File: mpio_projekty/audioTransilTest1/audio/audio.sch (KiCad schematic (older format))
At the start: 49 parts, among them J1 USB_B, J2 Mini-Fit Jr; 4,2mm, J3 TUEA4F2SOBHT, J4 Conn_02x05, J5 SWD_4pin, Q1 BC817, Q2 BC817, SW1 TACTM-34N-F, U1 STM32F042K6Tx, U2 AP1509-50SG-13, U3 LD1117S33TR, U4 IRLTS2242, U5 AO4616, U6 AO4616

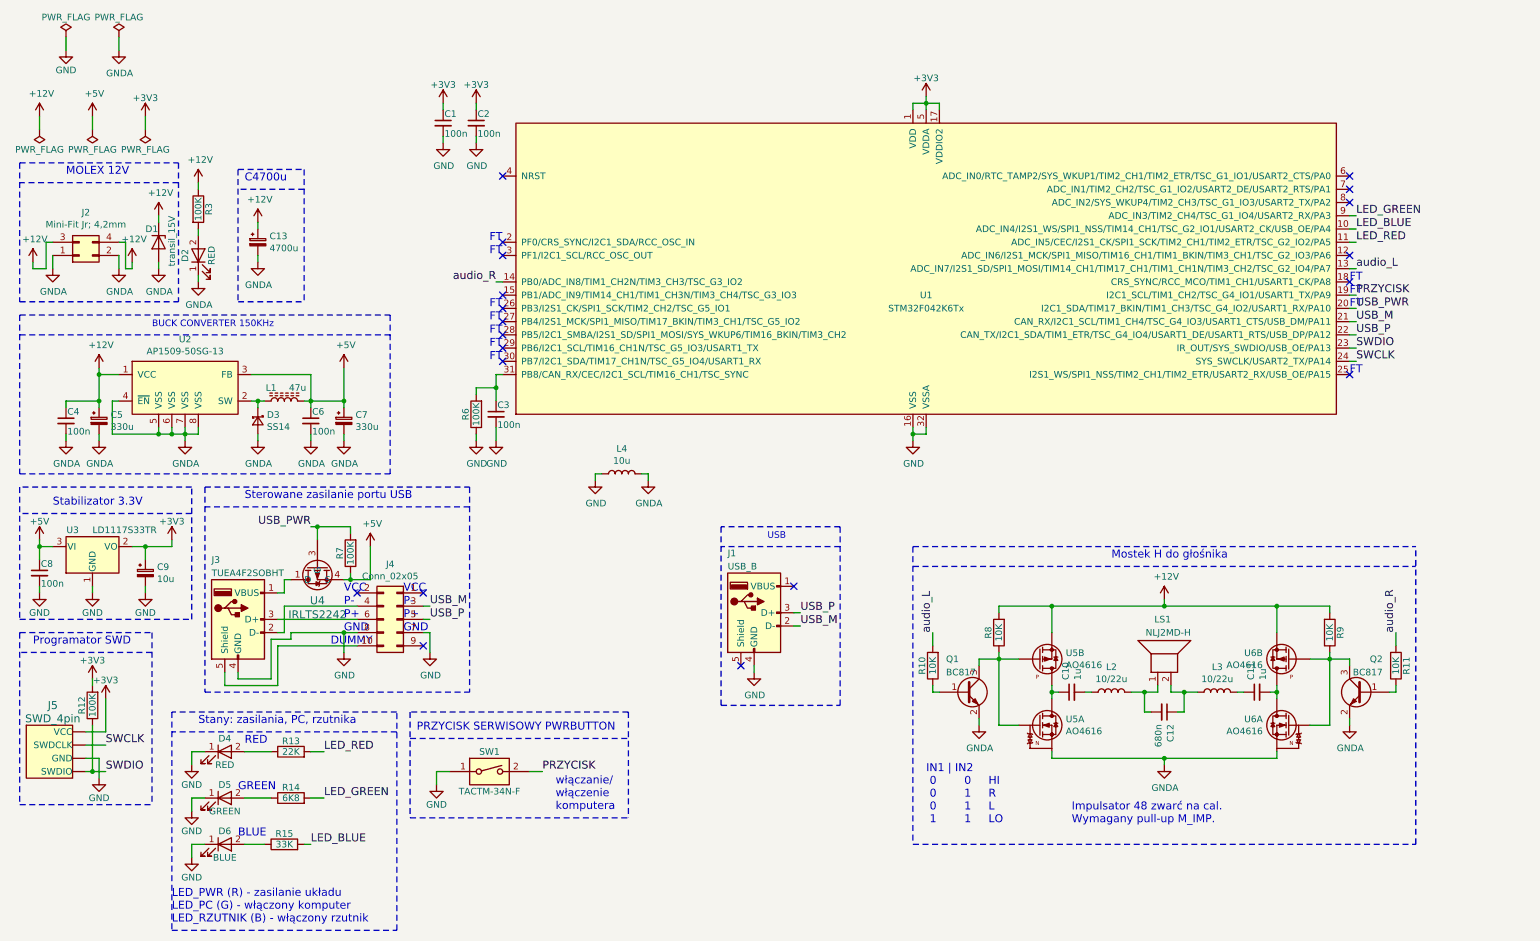
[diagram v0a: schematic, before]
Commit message: resetUSBv4.98com2
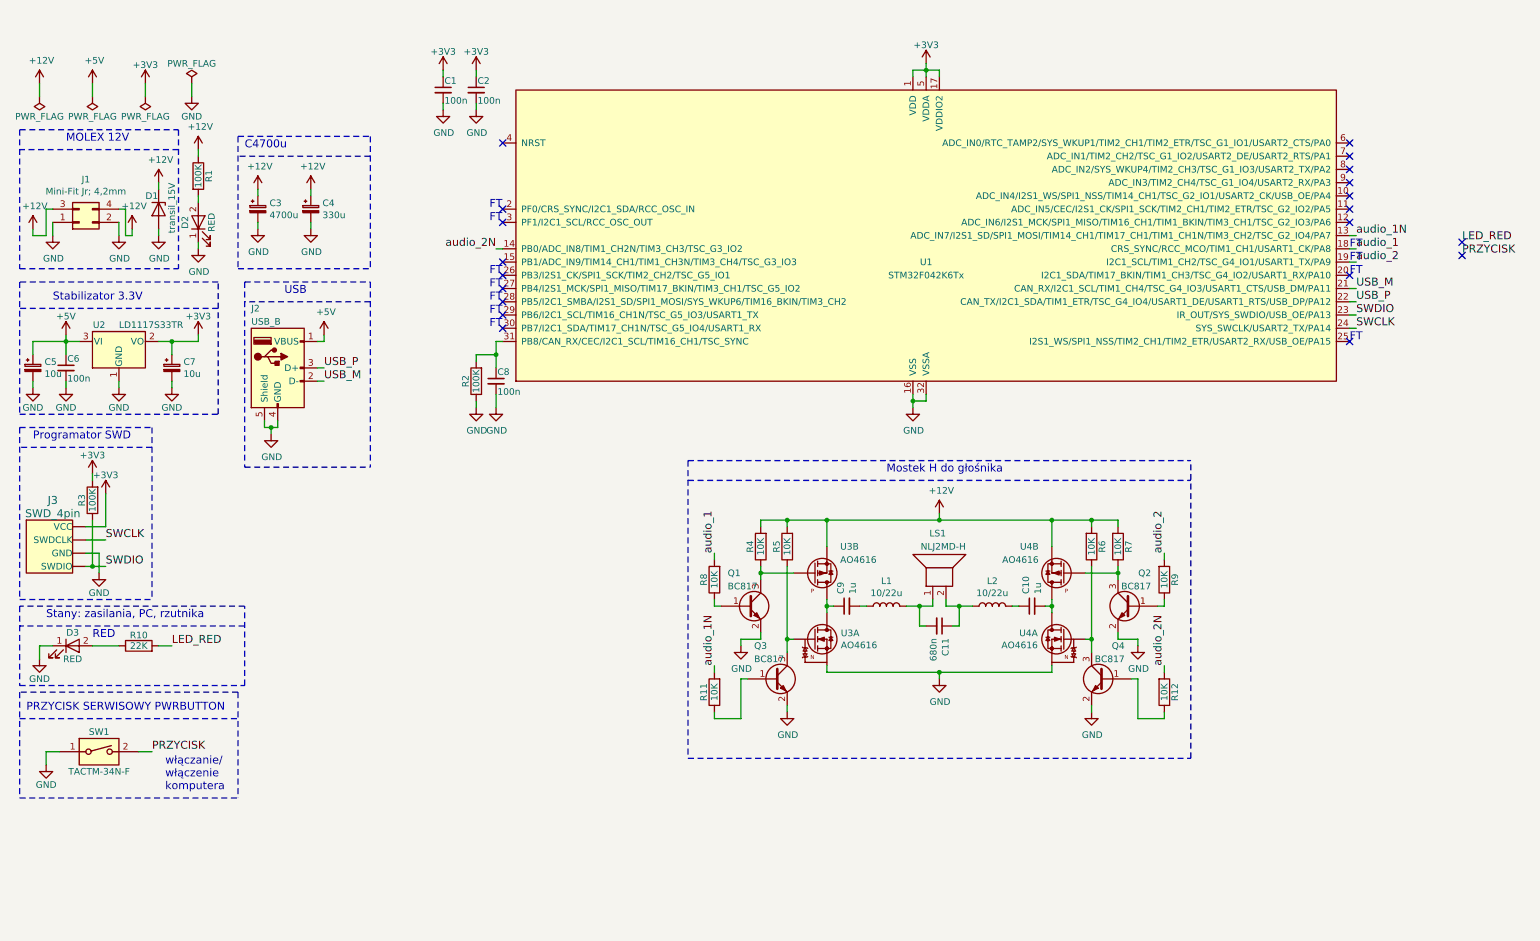
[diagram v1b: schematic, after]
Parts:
- removed C4, C6: 100n, Capacitors_SMD:C_0603, symbol device:C_Small
- removed C7: 330u, Capacitors_SMD:CP_Elec_10x10, symbol device:CP_Small
- removed D3: SS14, Diodes_SMD:D_SMA, symbol device:D_Schottky_Small
- removed D5: GREEN, LEDs:LED_0603, symbol device:LED
- removed D6: BLUE, LEDs:LED_0603, symbol device:LED
- removed J1: USB_B, mpio:USB_Micro-B, symbol conn:USB_A
- removed J4: Conn_02x05, mpio:IDC10, symbol conn:Conn_02x05_Odd_Even
- removed L1: 47u, Inductors_SMD:L_12x12mm_h6mm, symbol device:L_Core_Ferrite
- removed L4: 10u, Inductors_SMD:L_0805, symbol device:L
- removed R14: 6K8, Resistors_SMD:R_0603, symbol device:R
- removed R15: 33K, Resistors_SMD:R_0603, symbol device:R
- removed R7: 100K, Resistors_SMD:R_0603, symbol device:R
- removed U2: AP1509-50SG-13, Housings_SOIC:SOIC-8_3.9x4.9mm_Pitch1.27mm, symbol dc-dc:APE1707M-33-HF
- removed U4: IRLTS2242, mpio:TSOP-6_1.65x3.05mm_Pitch0.95mm, symbol mpio_lib:IRLTS2242
- added C4: 330u, Capacitors_THT:CP_Radial_D16.0mm_P7.50mm, symbol device:CP_Small
- added Q3, Q4: BC817, TO_SOT_Packages_SMD:SOT-23, symbol transistors:BC817
- added R11, R12, R5, R6: 10K, Resistors_SMD:R_0603, symbol device:R
- C5: value 330u -> 10u; footprint Capacitors_SMD:CP_Elec_8x6.5 -> Capacitors_SMD:CP_Elec_5x5.3
- J2: renamed from J3; value TUEA4F2SOBHT -> USB_B; footprint mpio:USB-A_SMD -> mpio:USB_Micro-B
- renumbered C11 to C10, C12 to C11, C13 to C3, C8 to C6, C9 to C7, C3 to C8, C10 to C9, D4 to D3, J2 to J1, J5 to J3, L2 to L1, L3 to L2, R3 to R1, R13 to R10, R6 to R2, R12 to R3, R8 to R4, R9 to R7, R10 to R8, R11 to R9, U3 to U2, U5 to U3, U6 to U4
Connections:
- net GNDA is gone; now on net GND: C3.2, C5.2, D1.2 (A), D2.1 (K), J1.1 (Pin_1), J1.2 (Pin_2), Q1.2 (E), Q2.2 (E), U3.1 (S), U4.1 (S)
- net +12V: now also C4.1, R5.2, R6.2; no longer C5.1
- net +5V: now also C5.1, J2.1 (VBUS)
- net GND: now also J2.5 (Shield), C4.2, Q3.2 (E), Q4.2 (E)
- net LED_RED: no longer U1.11 (ADC_IN5/CEC/I2S1_CK/SPI1_SCK/TIM2_CH1/TIM2_ETR/TSC_G2_IO2/PA5)
- net PRZYCISK: no longer U1.19 (I2C1_SCL/TIM1_CH2/TSC_G4_IO1/USART1_TX/PA9)
- net USB_M: now also J2.2 (D-)
- net USB_P: now also J2.3 (D+)
- net at Q1.3 (C), R4.1, U3.4 (G): no longer U3.2 (G)
- net at Q2.3 (C), R7.1, U4.4 (G): no longer U4.2 (G)
- net audio_1: now reaches U1.18 (CRS_SYNC/RCC_MCO/TIM1_CH1/USART1_CK/PA8)
- net audio_1: now also R8.2
- net LED_BLUE: no longer names the net of U1.10 (ADC_IN4/I2S1_WS/SPI1_NSS/TIM14_CH1/TSC_G2_IO1/USART2_CK/USB_OE/PA4)
- net LED_GREEN: no longer names the net of U1.9 (ADC_IN3/TIM2_CH4/TSC_G1_IO4/USART2_RX/PA3)
- net USB_PWR: no longer names the net of U1.20 (I2C1_SDA/TIM17_BKIN/TIM1_CH3/TSC_G4_IO2/USART1_RX/PA10)
- net audio_L renamed audio_1N
- net audio_1N: now also R11.2; no longer R8.2
- net audio_R renamed audio_2
- net audio_2: now also U1.19 (I2C1_SCL/TIM1_CH2/TSC_G4_IO1/USART1_TX/PA9); no longer U1.14 (PB0/ADC_IN8/TIM1_CH2N/TIM3_CH3/TSC_G3_IO2)
- new net: Q3.3 (C), R5.1, U3.2 (G)
- new net: Q4.3 (C), R6.1, U4.2 (G)
- new net: Q3.1 (B), R11.1
- new net: Q4.1 (B), R12.1
- new net audio_2N: R12.2, U1.14 (PB0/ADC_IN8/TIM1_CH2N/TIM3_CH3/TSC_G3_IO2)
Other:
- note removed: "BLUE"
- note removed: "BUCK CONVERTER 150KHz"
- note removed: "DUMMY"
- note removed: "GND"
- note removed: "GREEN"
- note removed: "IN1 | IN2\n 0 0 HI\n 0 1 R\n 0 1 L\n 1 1 LO"
- note removed: "Impulsator 48 zwarć na cal.\nWymagany pull-up M_IMP."
- note removed: "LED_PWR (R) - zasilanie układu\nLED_PC (G) - włączony komputer\nLED_RZUTNIK (B) - włączony rzutnik"
- note removed: "P+"
- note removed: "P-"
- note removed: "Sterowane zasilanie portu USB"
- note removed: "VCC"
- moved on the sheet: C1, C10, C11, C2, C3, C6, C7, C8, C9, D1, D2, D3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
